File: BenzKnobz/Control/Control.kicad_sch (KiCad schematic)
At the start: 98 parts, among them J1 Conn_01x02, J2 Conn_01x07, J3 Conn_01x07, J4 Conn_01x07, J5 Conn_01x07, J6 Conn_01x07, J7 Conn_01x07, J8 Conn_01x07, SW1 SW_MEC_5E, SW2 SW_MEC_5E, SW3 SW_MEC_5E, SW4 SW_MEC_5E, SW5 SW_MEC_5E, SW6 SW_MEC_5E

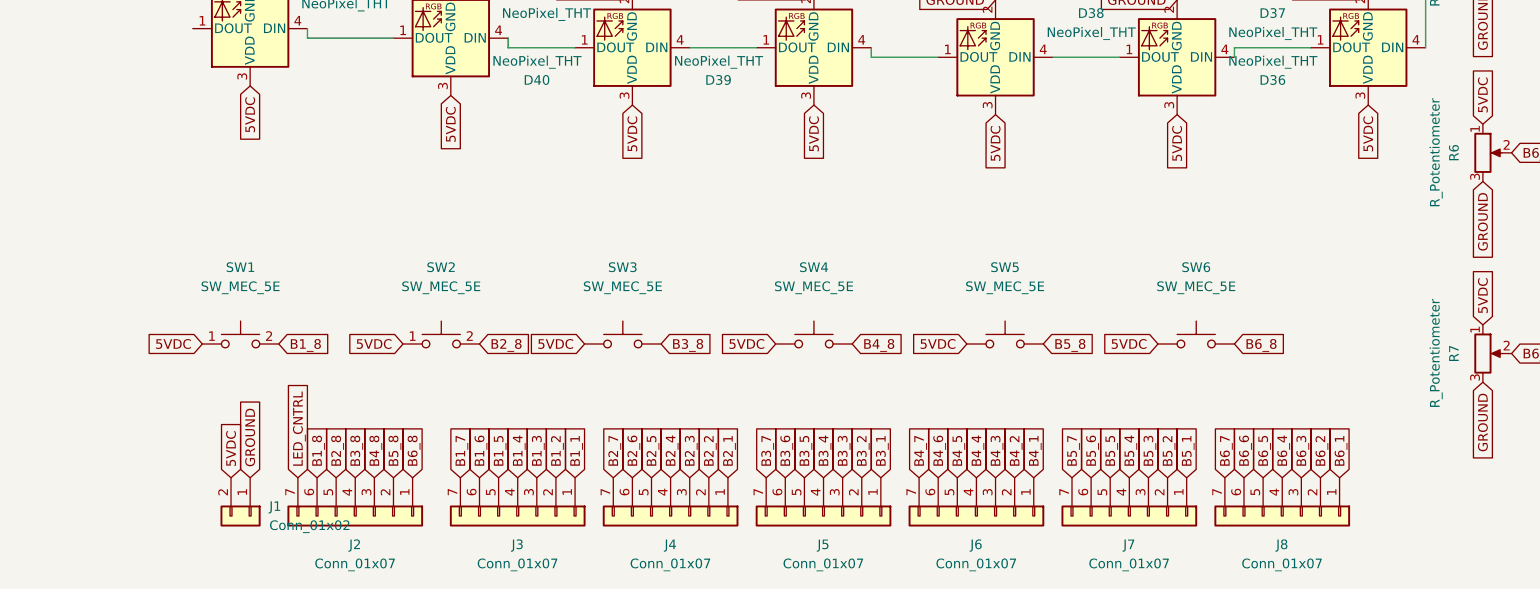
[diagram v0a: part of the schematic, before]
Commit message: brd
moar - almost completely laid out
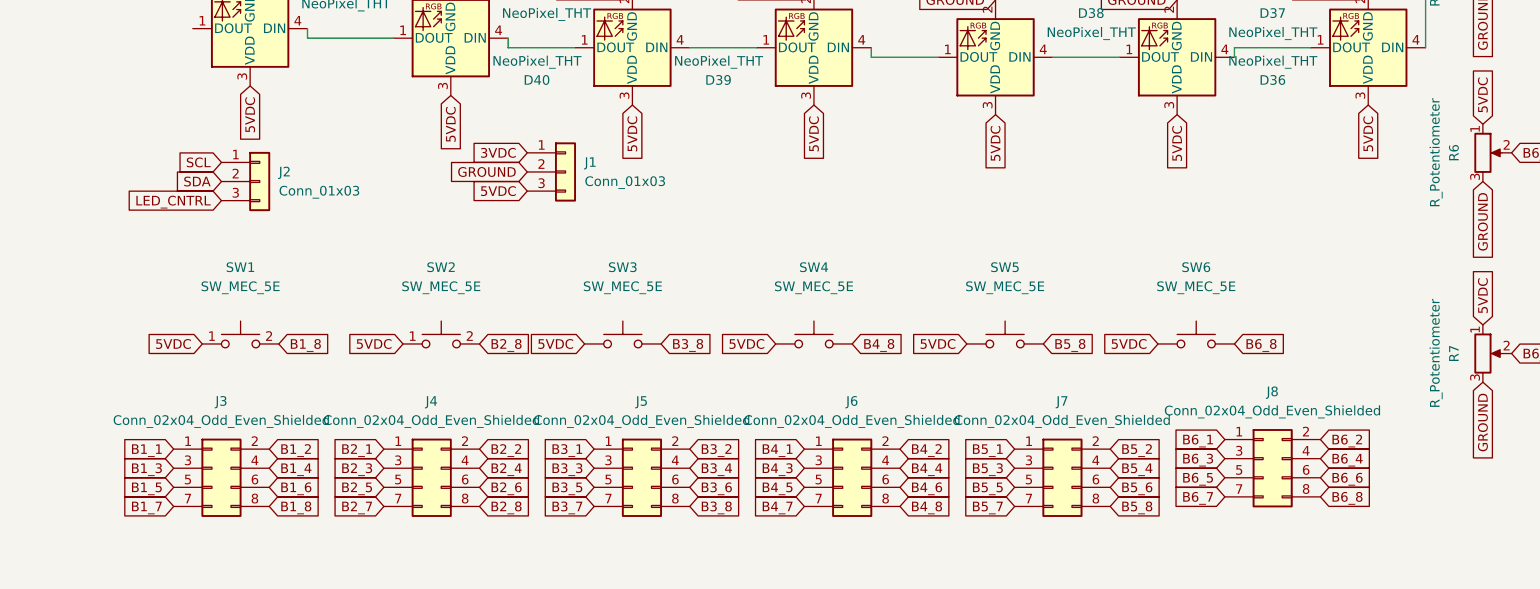
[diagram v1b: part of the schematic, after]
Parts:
- removed J1: Conn_01x02, Connector_PinHeader_1.00mm:PinHeader_1x02_P1.00mm_Vertical, symbol Connector_Generic:Conn_01x02
- removed J2, J3, J4, J5, J6, J7, J8: Conn_01x07, Connector_PinHeader_1.00mm:PinHeader_1x07_P1.00mm_Vertical, symbol Connector_Generic:Conn_01x07
- added J1, J2: Conn_01x03, Connector_PinHeader_1.00mm:PinHeader_1x03_P1.00mm_Vertical, symbol Connector_Generic:Conn_01x03
- added J3, J4, J5, J6, J7, J8: Conn_02x04_Odd_Even_Shielded, Connector_PinHeader_1.00mm:PinHeader_2x08_P1.00mm_Vertical, symbol Connector_Generic:Conn_02x04_Odd_Even
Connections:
- net 5VDC: now also J1.3 (Pin_3)
- net B1_1: now also J3.1 (Pin_1)
- net B1_2: now also J3.2 (Pin_2)
- net B1_3: now also J3.3 (Pin_3)
- net B1_4: now also J3.4 (Pin_4)
- net B1_5: now also J3.5 (Pin_5)
- net B1_6: now also J3.6 (Pin_6)
- net B1_7: now also J3.7 (Pin_7)
- net B1_8: now also J3.8 (Pin_8)
- net B2_1: now also J4.1 (Pin_1)
- net B2_2: now also J4.2 (Pin_2)
- net B2_3: now also J4.3 (Pin_3)
- net B2_4: now also J4.4 (Pin_4)
- net B2_5: now also J4.5 (Pin_5)
- net B2_6: now also J4.6 (Pin_6)
- net B2_7: now also J4.7 (Pin_7)
- net B2_8: now also J4.8 (Pin_8)
- net B3_1: now also J5.1 (Pin_1)
- net B3_2: now also J5.2 (Pin_2)
- net B3_3: now also J5.3 (Pin_3)
- net B3_4: now also J5.4 (Pin_4)
- net B3_5: now also J5.5 (Pin_5)
- net B3_6: now also J5.6 (Pin_6)
- net B3_7: now also J5.7 (Pin_7)
- net B3_8: now also J5.8 (Pin_8)
- net B4_1: now also J6.1 (Pin_1)
- net B4_2: now also J6.2 (Pin_2)
- net B4_3: now also J6.3 (Pin_3)
- net B4_4: now also J6.4 (Pin_4)
- net B4_5: now also J6.5 (Pin_5)
- net B4_6: now also J6.6 (Pin_6)
- net B4_7: now also J6.7 (Pin_7)
- net B4_8: now also J6.8 (Pin_8)
- net B5_1: now also J7.1 (Pin_1)
- net B5_2: now also J7.2 (Pin_2)
- net B5_3: now also J7.3 (Pin_3)
- net B5_4: now also J7.4 (Pin_4)
- net B5_5: now also J7.5 (Pin_5)
- net B5_6: now also J7.6 (Pin_6)
- net B5_7: now also J7.7 (Pin_7)
- net B5_8: now also J7.8 (Pin_8)
- net B6_1: now also J8.1 (Pin_1)
- net B6_2: now also J8.2 (Pin_2)
- net B6_3: now also J8.3 (Pin_3)
- net B6_4: now also J8.4 (Pin_4)
- net B6_5: now also J8.5 (Pin_5)
- net B6_6: now also J8.6 (Pin_6)
- net B6_7: now also J8.7 (Pin_7)
- net B6_8: now also J8.8 (Pin_8)
- net GROUND: now also J1.2 (Pin_2)
- net LED_CNTRL: now also J2.3 (Pin_3)
- new net 3VDC: J1.1 (Pin_1)
- new net SCL: J2.1 (Pin_1)
- new net SDA: J2.2 (Pin_2)
